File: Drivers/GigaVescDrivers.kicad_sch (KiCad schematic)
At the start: 15 parts, among them J1 LogicConn, U8 74LVC1G125GV,125

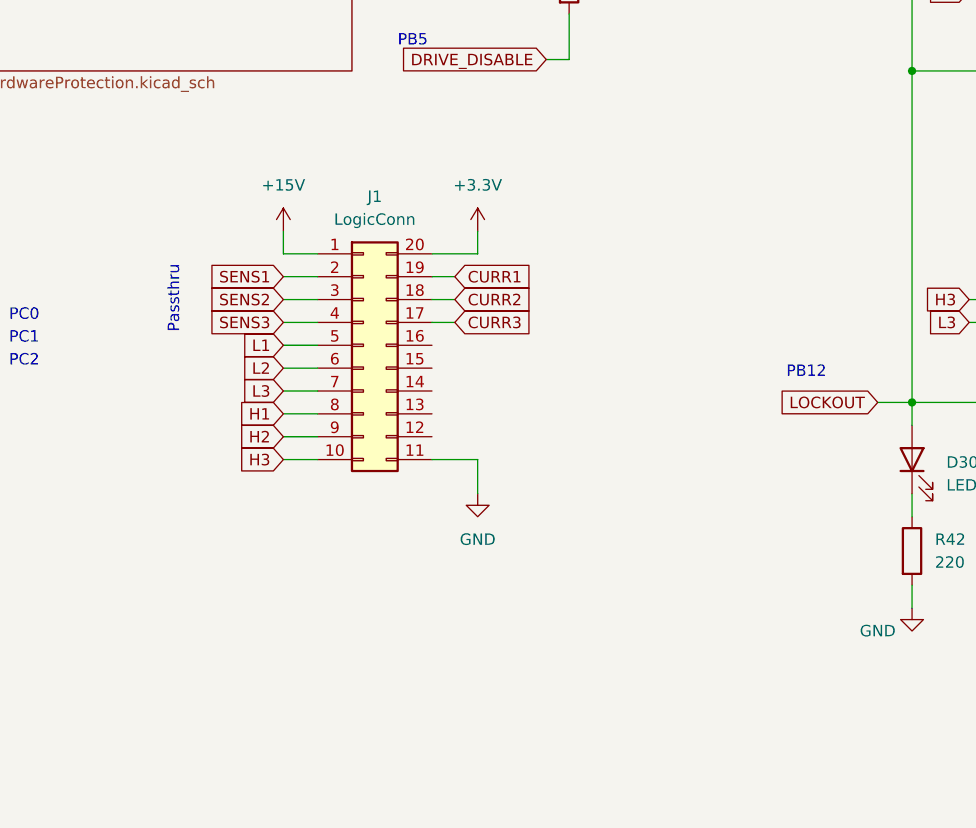
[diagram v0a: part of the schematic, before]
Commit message: initial
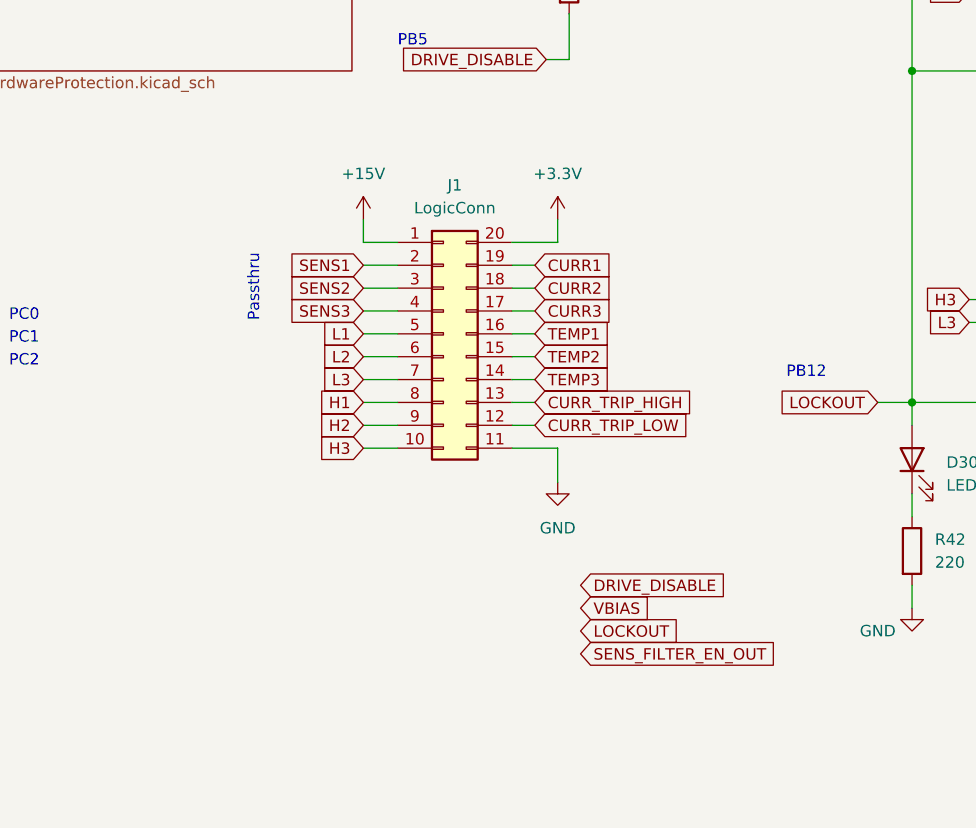
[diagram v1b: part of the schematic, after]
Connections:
- net CURR_TRIP_HIGH: now also J1.13 (Pin_13)
- net CURR_TRIP_LOW: now also J1.12 (Pin_12)
- net TEMP1: now also J1.16 (Pin_16)
- net TEMP2: now also J1.15 (Pin_15)
- net TEMP3: now also J1.14 (Pin_14)
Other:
- moved on the sheet: J1
